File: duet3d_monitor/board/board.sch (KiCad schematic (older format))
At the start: 15 parts, among them J1 Connector_01x04_Male, J2 Connector_01x04_Male, J3 Connector_01x03_Male, J4 Screw_Terminal_x02, U1 Teensy-LC, U2 TBA 2-2411

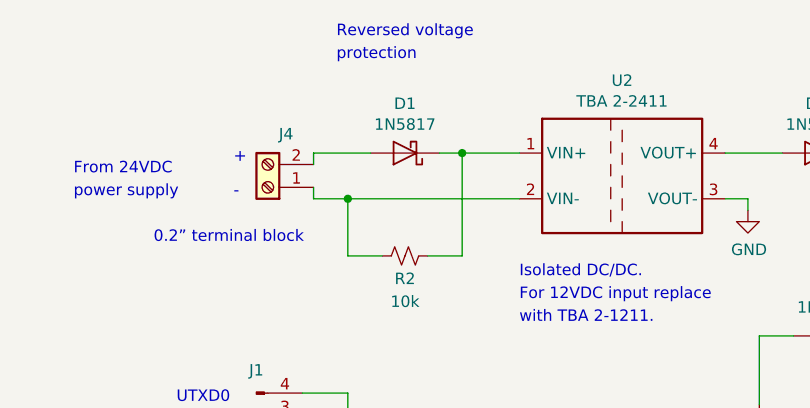
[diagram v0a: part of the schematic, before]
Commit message: Minor schematic tweaks
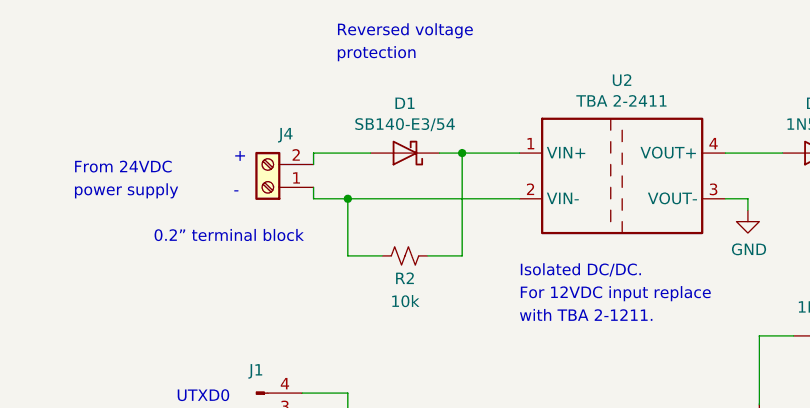
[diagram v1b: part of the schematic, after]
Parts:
- D1: value 1N5817 -> SB140-E3/54
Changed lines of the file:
@@
 P 3350 2250
 F 0 "D1" H 3350 2034 50  0000 C CNN
-F 1 "1N5817" H 3350 2125 50  0000 C CNN
+F 1 "SB140-E3/54" H 3350 2125 50  0000 C CNN
 F 2 "board:Diode" H 3350 2075 50  0001 C CNN
 F 3 "http://www.vishay.com/docs/88525/1n5817.pdf" H 3350 2250 50  0001 C CNN

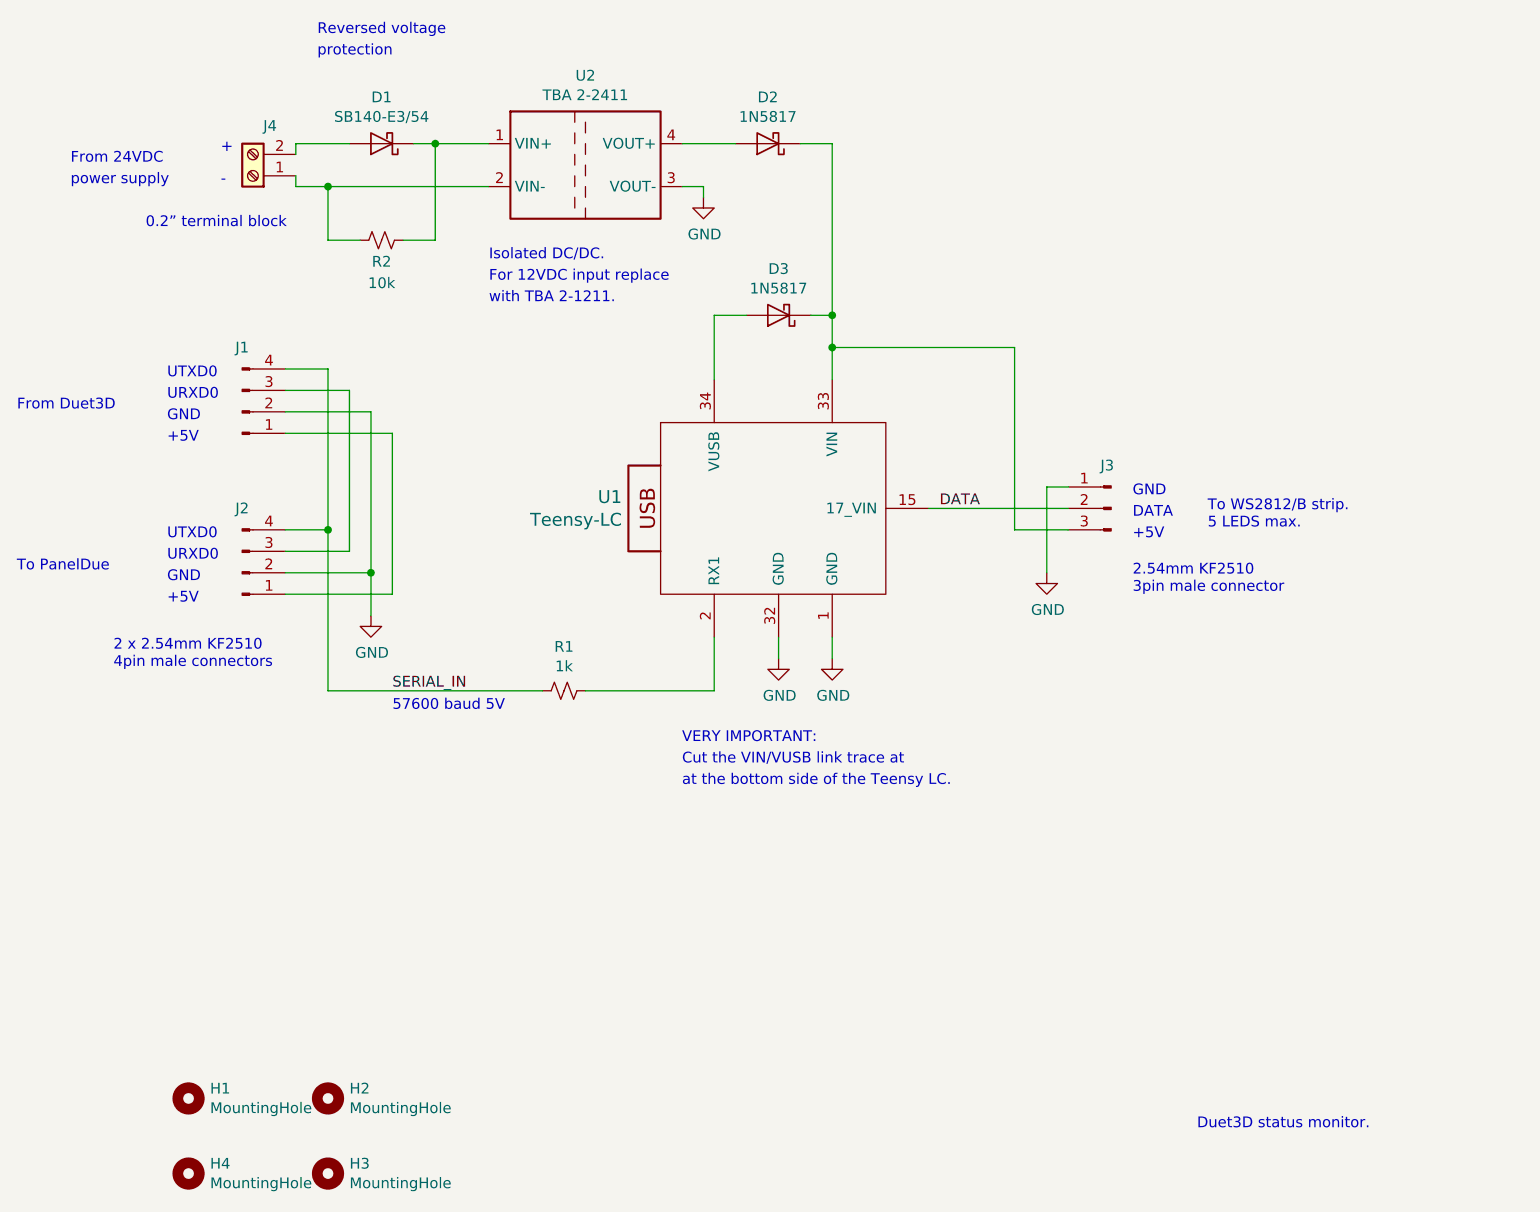
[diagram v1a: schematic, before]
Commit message: Flushing misc/repo changes.
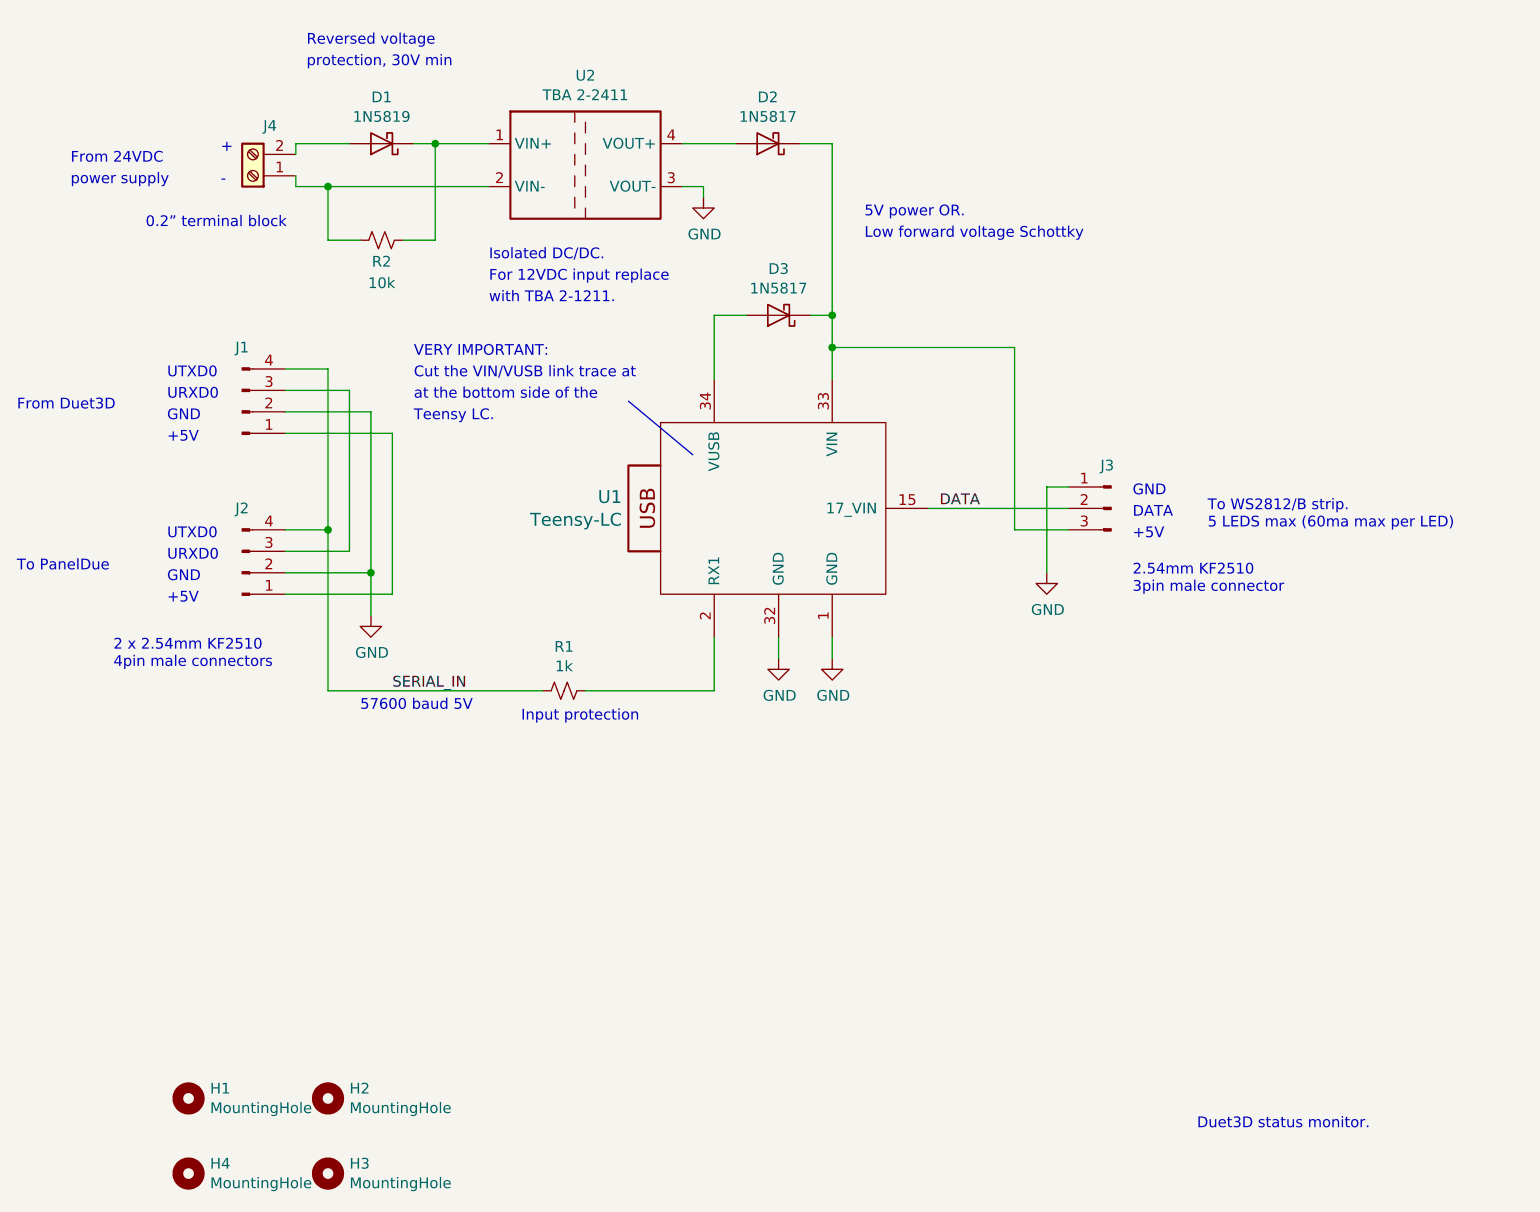
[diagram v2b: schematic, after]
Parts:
- D1: value SB140-E3/54 -> 1N5819
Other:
- note added: "5V power OR."
- note added: "Input protection"
- note added: "Low forward voltage Schottky"
- note added: "Teensy LC."
- note added: "To WS2812/B strip.\n5 LEDS max (60ma max per LED)"
- note added: "\nprotection, 30V min"
- note added: "at the bottom side of the"
- note removed: "To WS2812/B strip.\n5 LEDS max."
- note removed: "\nprotection"
- note removed: "at the bottom side of the Teensy LC."
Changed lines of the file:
@@
 with TBA 2-1211.
 Text Notes 7200 4050 0    50   ~ 0
-To WS2812/B strip.\n5 LEDS max.
-Text Notes 4750 5050 0    50   ~ 0
+To WS2812/B strip.\n5 LEDS max (60ma max per LED)
+Text Notes 3500 3250 0    50   ~ 0
 VERY IMPORTANT:
 Text Notes 1650 4250 0    50   ~ 0
 To PanelDue
-Text Notes 4750 5150 0    50   ~ 0
+Text Notes 3500 3350 0    50   ~ 0
 Cut the VIN/VUSB link trace at
-Text Notes 4750 5250 0    50   ~ 0
-at the bottom side of the Teensy LC.
-Text Notes 3050 1750 0    50   ~ 0
+Text Notes 3500 3450 0    50   ~ 0
+at the bottom side of the
+Text Notes 3000 1800 0    50   ~ 0
 Reversed voltage
-Text Notes 3050 1850 0    50   ~ 0
-\nprotection
+Text Notes 3000 1900 0    50   ~ 0
+\nprotection, 30V min
 Text Notes 1650 3500 0    50   ~ 0
 From Duet3D
@@
 Text Notes 1900 2450 0    50   ~ 0
 power supply
-Text Notes 3400 4900 0    50   ~ 0
+Text Notes 3250 4900 0    50   ~ 0
 57600 baud 5V
 Text Notes 3850 2800 0    50   ~ 0
@@
 P 3350 2250
 F 0 "D1" H 3350 2034 50  0000 C CNN
-F 1 "SB140-E3/54" H 3350 2125 50  0000 C CNN
+F 1 "1N5819" H 3350 2125 50  0000 C CNN
 F 2 "board:Diode" H 3350 2075 50  0001 C CNN
 F 3 "http://www.vishay.com/docs/88525/1n5817.pdf" H 3350 2250 50  0001 C CNN
@@
 Wire Wire Line
 	6450 3850 6450 4250
+Text Notes 5600 2600 0    50   ~ 0
+5V power OR.
+Text Notes 5600 2700 0    50   ~ 0
+Low forward voltage Schottky
+Text Notes 4000 4950 0    50   ~ 0
+Input protection
+Wire Bus Line
+	4800 3700 4500 3450
+Text Notes 3500 3550 0    50   ~ 0
+Teensy LC.
 $EndSCHEMATC
